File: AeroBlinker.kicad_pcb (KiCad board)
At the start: 2 copper layers, 41.8 x 28 mm, 33 parts, among them J1 LED_GND, J2 LED_GND, J3 LED_GND, J4 BATTERY, J5 RECEIVER, J6 USB_C_Receptacle_USB2.0_16P, Q1 AO3400A, SW2 SW_Push, U1 STM32F042F6Px, U2 USBLC6-2SC6, U3 TPS62162DGR

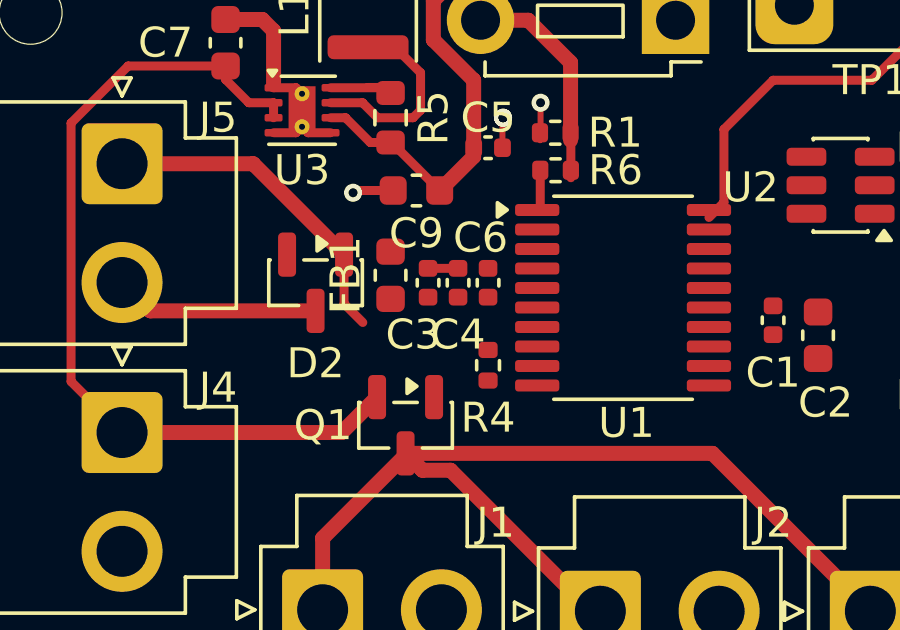
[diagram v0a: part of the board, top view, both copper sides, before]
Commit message: Autosave
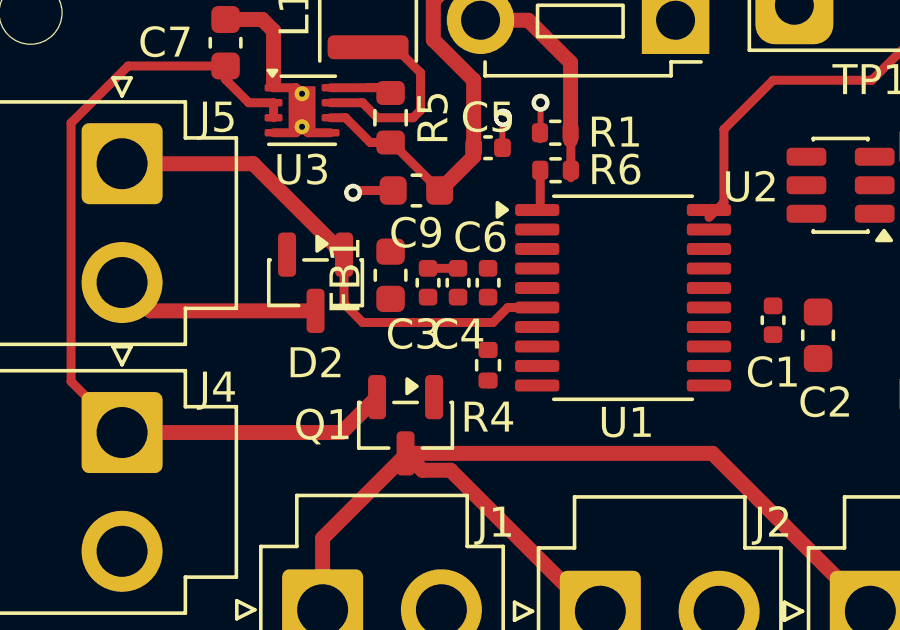
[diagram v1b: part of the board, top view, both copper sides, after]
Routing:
- net RECV_PWM: track 11.2 -> 17.2 mm
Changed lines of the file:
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@@
+	)
+	(segment
+		(start 138.325 131.075)
+		(end 142.661846 131.075)
+		(width 0.3)
+		(layer "F.Cu")
+		(net "RECV_PWM")
+	)
+	(segment
+		(start 142.661846 131.075)
+		(end 143.161846 130.575)
+		(width 0.3)
+		(layer "F.Cu")
+		(net "RECV_PWM")
 	)
 	(segment
@@
 		(layer "F.Cu")
 		(net "RECV_PWM")
+	)
+	(segment
+		(start 143.161846 130.575)
+		(end 144.1375 130.575)
+		(width 0.3)
+		(layer "F.Cu")
+		(net "RECV_PWM")

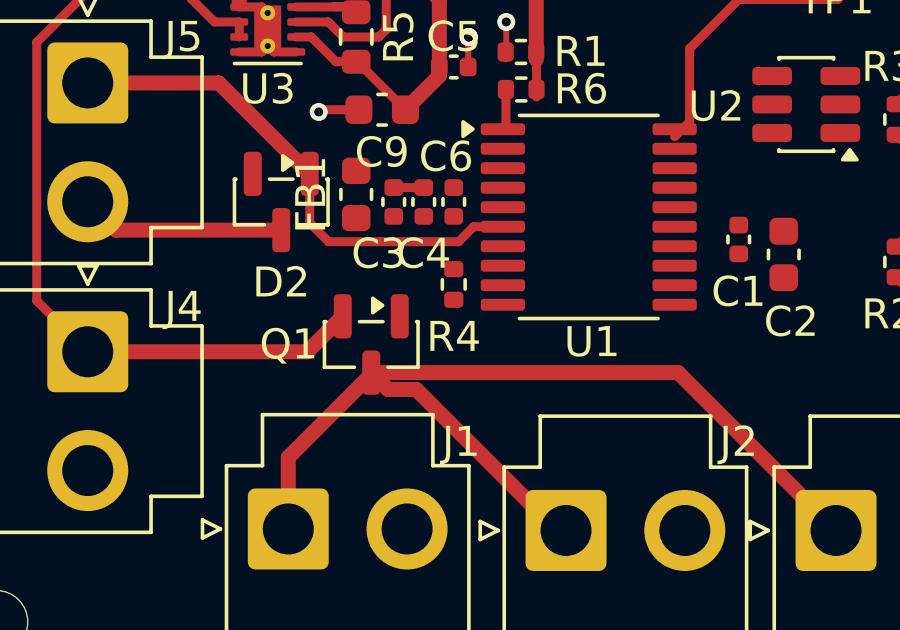
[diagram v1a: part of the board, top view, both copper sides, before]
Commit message: Autosave
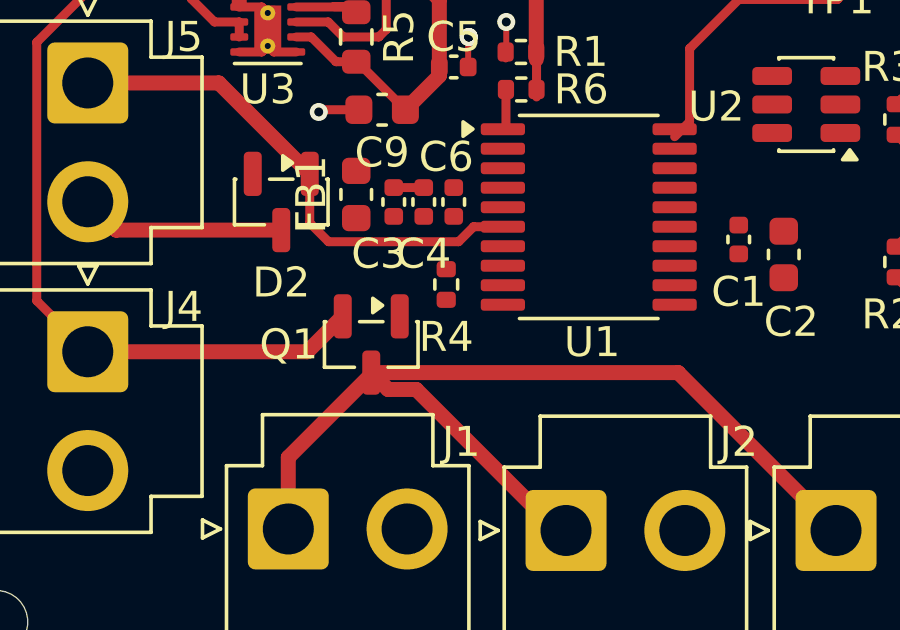
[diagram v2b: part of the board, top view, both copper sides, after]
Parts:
- moved R4 0.25 mm to (142.2, 132.5)
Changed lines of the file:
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@@
 	(footprint "Resistor_SMD:R_0402_1005Metric"
 		(layer "F.Cu")
-		(at 142.5 132.5 90)
+		(at 142.25 132.5 90)
 		(descr "Resistor SMD 0402 (1005 Metric), square (rectangular) end terminal, IPC-7351 nominal, (Body size source: IPC-SM-782 page 72, https://www.pcb-3d.com/wordpress/wp-content/uploads/ipc-sm-782a_amendment_1_and_2.pdf)")
 		(tags "resistor")

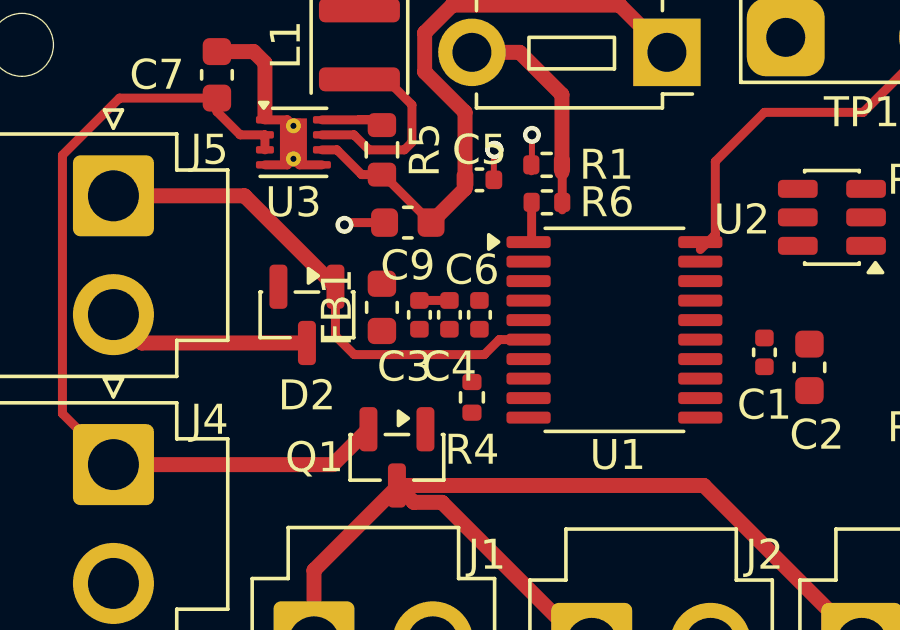
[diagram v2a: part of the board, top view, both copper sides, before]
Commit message: Autosave
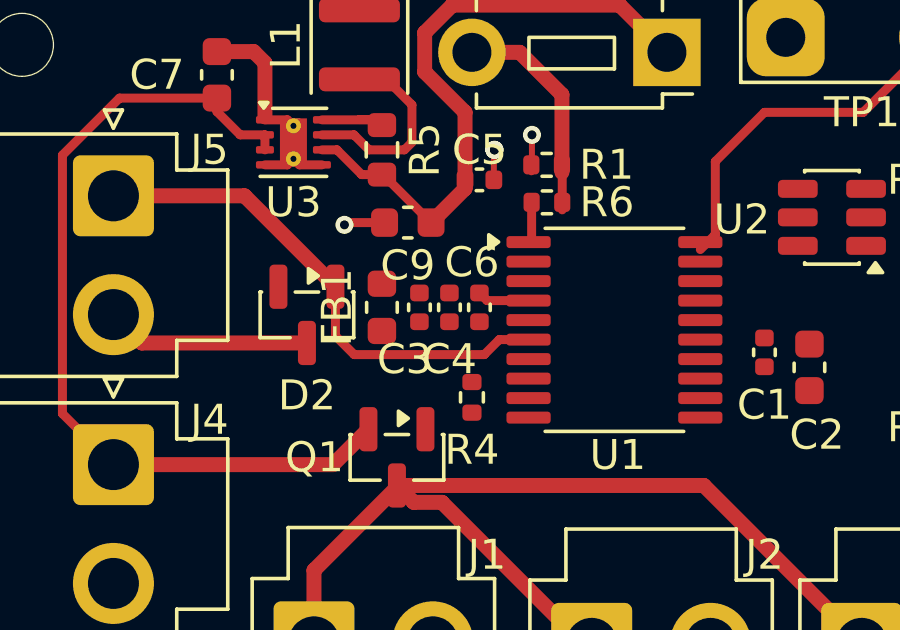
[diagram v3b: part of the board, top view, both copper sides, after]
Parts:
- moved C3 0.25 mm to (140.5, 129.5)
- moved C4 0.25 mm to (141.5, 129.5)
- moved C6 0.25 mm to (142.5, 129.5)
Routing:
- net /NRST: track 0.00 -> 1.74 mm
- net GND: track 17.7 -> 16.7 mm
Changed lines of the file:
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@@
 	(footprint "Capacitor_SMD:C_0402_1005Metric"
 		(layer "F.Cu")
-		(at 142.5 129.75 -90)
+		(at 142.5 129.5 -90)
 		(descr "Capacitor SMD 0402 (1005 Metric), square (rectangular) end terminal, IPC-7351 nominal, (Body size source: IPC-SM-782 page 76, https://www.pcb-3d.com/wordpress/wp-content/uploads/ipc-sm-782a_amendment_1_and_2.pdf)")
 		(tags "capacitor")
@@
 	(footprint "Capacitor_SMD:C_0402_1005Metric"
 		(layer "F.Cu")
-		(at 141.5 129.75 90)
+		(at 141.5 129.5 90)
 		(descr "Capacitor SMD 0402 (1005 Metric), square (rectangular) end terminal, IPC-7351 nominal, (Body size source: IPC-SM-782 page 76, https://www.pcb-3d.com/wordpress/wp-content/uploads/ipc-sm-782a_amendment_1_and_2.pdf)")
 		(tags "capacitor")
@@
 	(footprint "Capacitor_SMD:C_0402_1005Metric"
 		(layer "F.Cu")
-		(at 140.5 129.75 90)
+		(at 140.5 129.5 90)
 		(descr "Capacitor SMD 0402 (1005 Metric), square (rectangular) end terminal, IPC-7351 nominal, (Body size source: IPC-SM-782 page 76, https://www.pcb-3d.com/wordpress/wp-content/uploads/ipc-sm-782a_amendment_1_and_2.pdf)")
 		(tags "capacitor")
@@
 	)
 	(segment
-		(start 141.5 129.27)
-		(end 140.5 129.27)
-		(width 0.3)
-		(layer "F.Cu")
-		(net "GND")
-	)
-	(segment
 		(start 159.07 126.3)
 		(end 159.07 125.755)
@@
 	)
 	(segment
+		(start 142.5 129.02)
+		(end 142.755 129.275)
+		(width 0.3)
+		(layer "F.Cu")
+		(net "/NRST")
+	)
+	(segment
+		(start 142.755 129.275)
+		(end 144.1375 129.275)
+		(width 0.3)
+		(layer "F.Cu")
+		(net "/NRST")
+	)
+	(segment

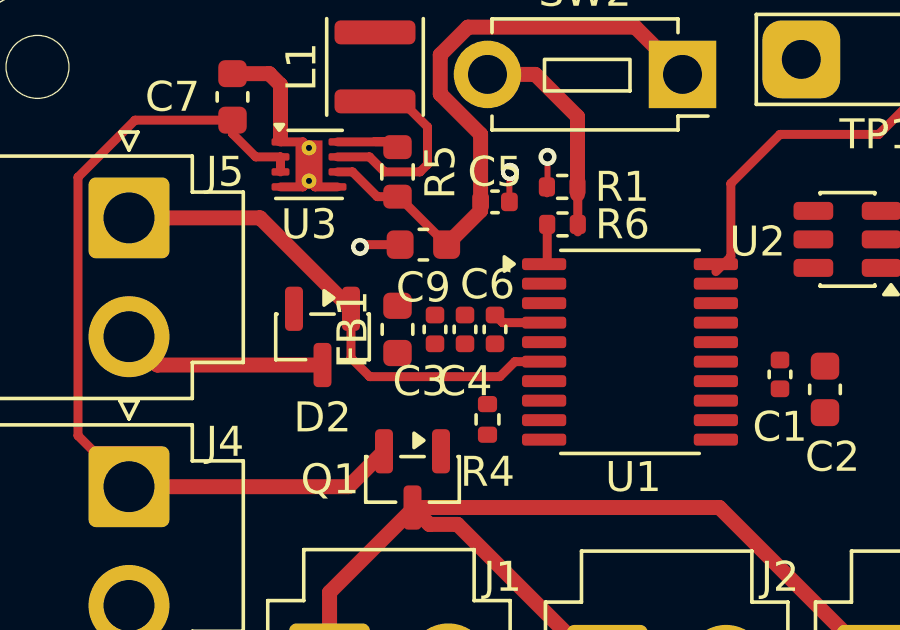
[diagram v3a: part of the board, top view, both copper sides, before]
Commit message: Autosave
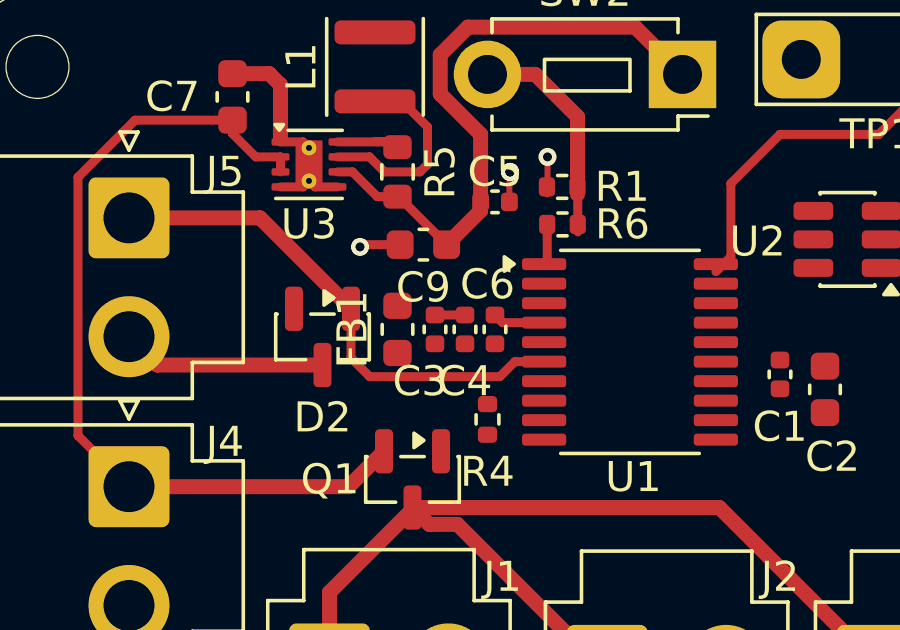
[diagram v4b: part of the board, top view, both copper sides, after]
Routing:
- net GND: track 16.7 -> 17.7 mm
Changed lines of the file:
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@@
+	)
+	(segment
+		(start 140.5 129.02)
+		(end 141.5 129.02)
+		(width 0.3)
+		(layer "F.Cu")
+		(net "GND")
 	)
 	(segment
